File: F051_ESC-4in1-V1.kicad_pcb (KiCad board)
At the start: 4 copper layers, 46 x 55.8 mm, 222 parts, among them J1 Conn_01x02, J11 Conn_01x03, J14 Conn_01x03, J2 Conn_01x10, J3 Conn_01x05, J4 Conn_01x05, J5 Conn_01x05, J6 Conn_01x03, J7 Conn_01x05, J8 Conn_01x03, J9 Conn_01x10, Q1 TPHR8504PL, Q10 TPHR8504PL, Q11 TPHR8504PL, Q12 TPHR8504PL, Q13 TPHR8504PL, Q14 TPHR8504PL, Q15 TPHR8504PL, Q16 TPHR8504PL, Q17 TPHR8504PL, Q18 TPHR8504PL, Q19 TPHR8504PL, Q2 TPHR8504PL, Q20 TPHR8504PL, Q21 TPHR8504PL, Q22 TPHR8504PL, Q23 TPHR8504PL, Q24 TPHR8504PL, Q3 TPHR8504PL, Q4 TPHR8504PL, Q5 TPHR8504PL, Q6 TPHR8504PL, Q7 TPHR8504PL, Q8 TPHR8504PL, Q9 TPHR8504PL, U1 STM32F051K6Ux, U10 FD6288Q, U11 STM32F051K6Ux, U12 FD6288Q, U13 L78L12_SOT89, U14 MP4560_QFN10, U2 FD6288Q, U3 L78L12_SOT89, U4 LP2985-3.3, U5 INA139, U6 FD6288Q, U7 OPA340NA, U8 STM32F051K6Ux, U9 STM32F051K6Ux

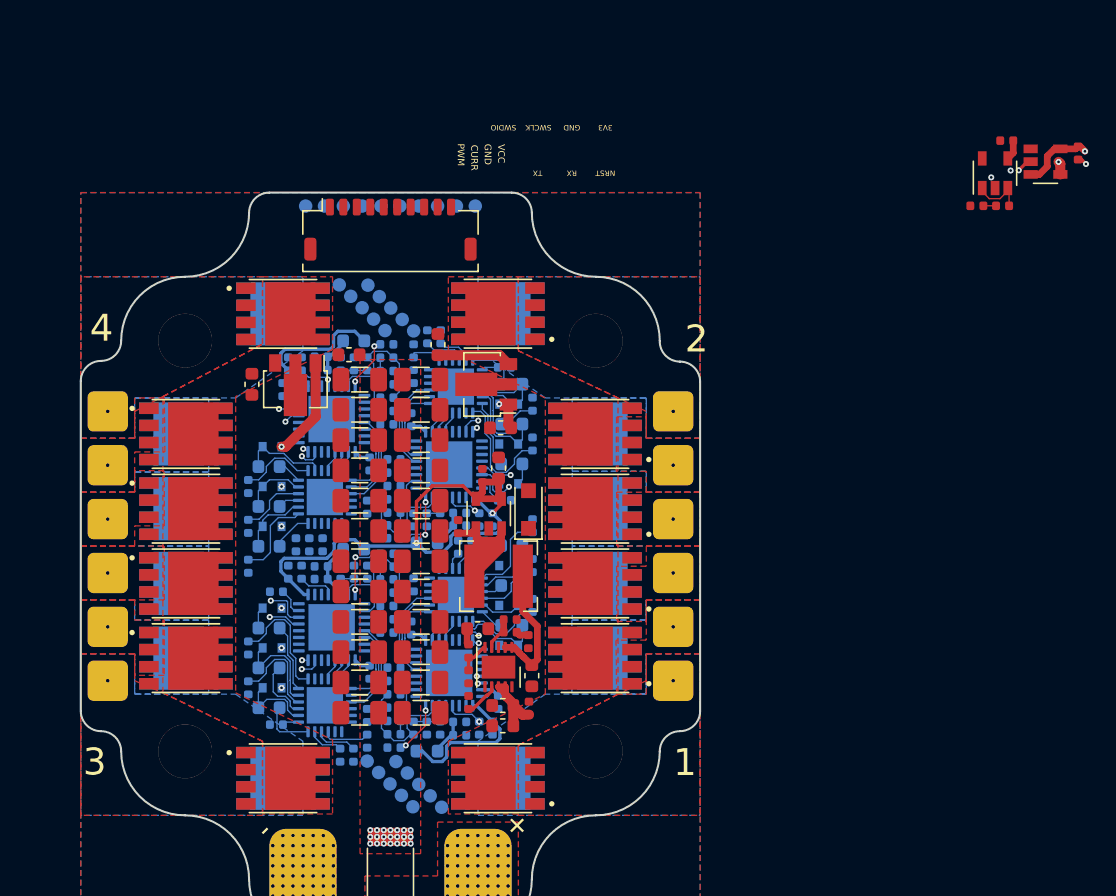
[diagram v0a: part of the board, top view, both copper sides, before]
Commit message: Connected a lot of stuff
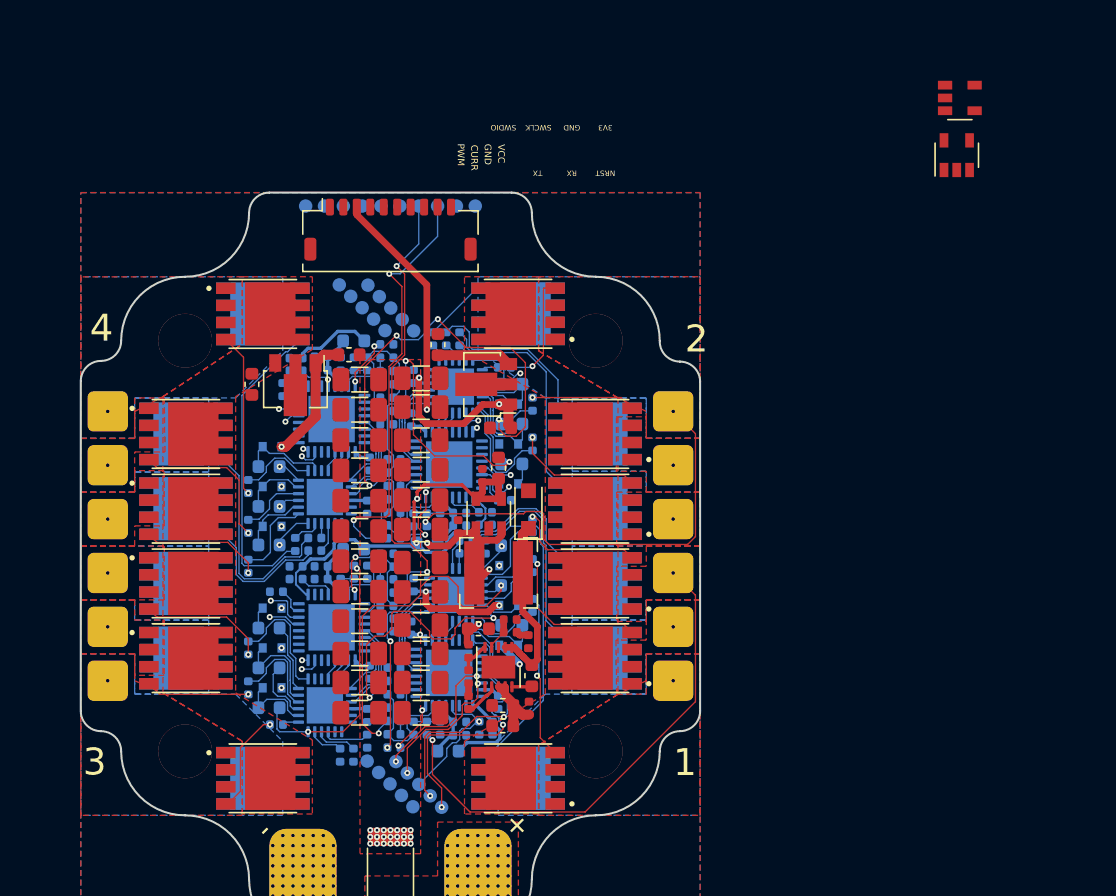
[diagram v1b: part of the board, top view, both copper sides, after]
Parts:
- removed C7: 0.1uF, Capacitor_SMD:C_0402_1005Metric
- removed C8: 3.3nF, Capacitor_SMD:C_0402_1005Metric
- removed R2: 60k, Resistor_SMD:R_0402_1005Metric
- removed R3: 500, Resistor_SMD:R_0402_1005Metric
- moved U5 7.93 mm to (182.3, 55.2)
- moved U7 3.14 mm to (182.1, 59.5)
- moved R26 1.69 mm to (143.2, 73.1)
- moved FB1 1.55 mm to (144.3, 103.7), turned to 0 degrees
- moved Q1 1.50 mm to (149.5, 105.8)
- moved Q11 1.50 mm to (149.5, 71.2)
- moved Q12 1.50 mm to (149.5, 71.2)
- moved Q17 1.50 mm to (130.5, 105.8)
- moved Q18 1.50 mm to (130.5, 105.8)
- moved Q19 1.50 mm to (130.5, 71.3)
- moved Q2 1.50 mm to (149.5, 105.8)
- moved Q20 1.50 mm to (130.5, 71.3)
- moved R5 1.41 mm to (145.1, 73.1)
- moved R22 1.41 mm to (144.1, 73.1)
- moved R24 0.75 mm to (145.6, 88.1), turned to 180 degrees
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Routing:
- net /MCU 2/PhaseB: track 4.49 -> 55.8 mm, vias 0 -> 4
- net /MCU 1/PhaseC: track 3.37 -> 54.5 mm, vias 0 -> 2
- net /MCU 2/PhaseC: track 4.74 -> 52.1 mm, vias 0 -> 2
- net /PWM_1: track 0.00 -> 45.7 mm, vias 0 -> 4
- net /MCU 1/PhaseB: track 1.59 -> 40.8 mm, vias 0 -> 2
- net /MCU 2/PhaseA: track 5.46 -> 43.7 mm, vias 0 -> 2
- net /MCU 1/PhaseA: track 1.82 -> 36.6 mm, vias 0 -> 2
- net /PWM_2: track 0.00 -> 31.8 mm, vias 0 -> 2
- net +5V: track 18.1 -> 48.0 mm, vias 0 -> 4
- net +12V: track 9.26 -> 37.4 mm, vias 7 -> 12
- net Net-(Q2-Pad4): track 0.00 -> 23.7 mm
- net Net-(Q20-Pad4): track 0.00 -> 23.0 mm
- net /MCU 1/SWCLK: track 0.54 -> 20.6 mm, vias 1 -> 2
- net /MCU 1/SWDIO: track 1.62 -> 19.8 mm, vias 1 -> 2
- net Net-(Q8-Pad4): track 0.00 -> 16.6 mm
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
